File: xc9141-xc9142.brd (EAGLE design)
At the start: 13.6 x 21.6 mm, 7 parts

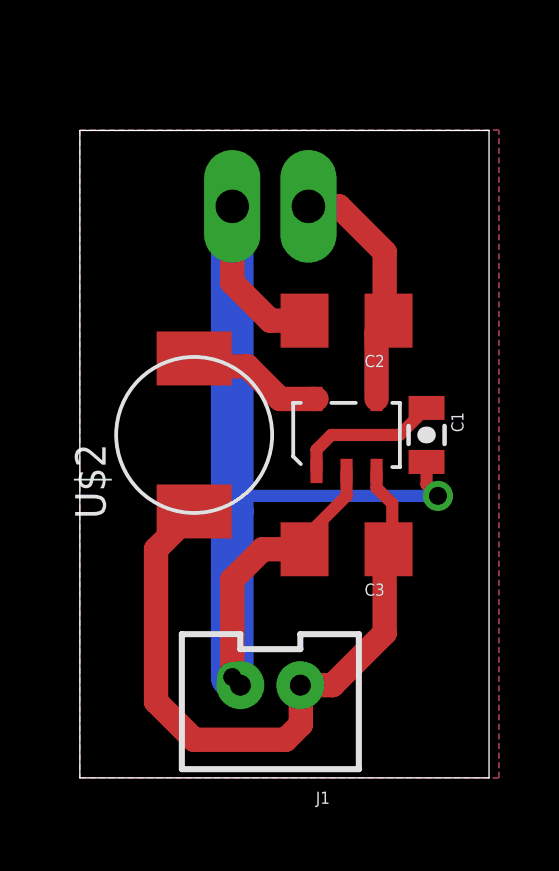
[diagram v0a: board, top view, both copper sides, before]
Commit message: Breakout board updates
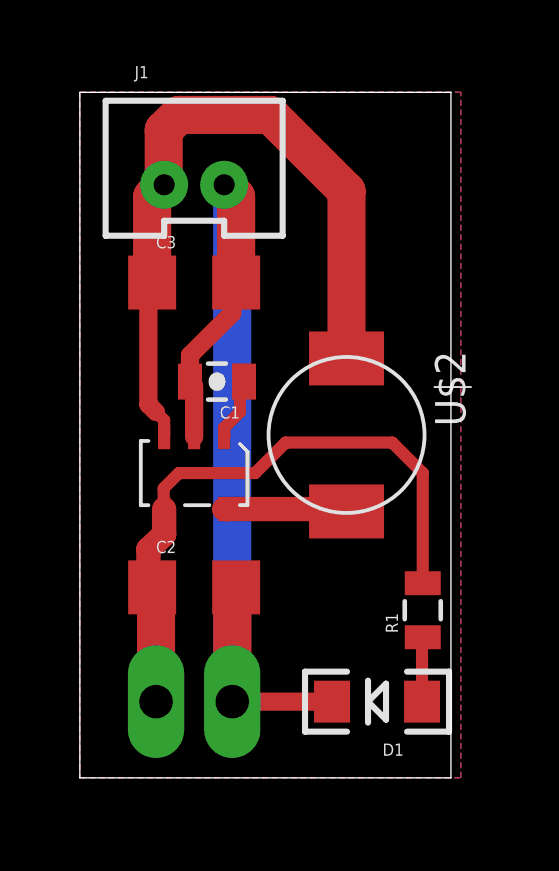
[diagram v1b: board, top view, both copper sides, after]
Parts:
- added D1: YELLOW, SparkFun-LED:LED-1206
- added R1: 680, SparkFun-Resistors:0805
- moved J1 18.0 mm to (3.81, 20.3), turned to 0 degrees
- moved J2 17.3 mm to (2.54, 2.54), turned to 0 degrees
- moved C2 10.2 mm to (3.81, 6.35), turned to 0 degrees
- moved C3 10.2 mm to (3.81, 16.5), turned to 0 degrees
- moved C1 7.21 mm to (4.57, 13.2), turned to 180 degrees
- moved U$1 5.24 mm to (3.81, 10.2), turned to 180 degrees
- moved U$2 5.08 mm to (8.89, 11.4), turned to 270 degrees
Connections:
- new net N$1: D1.A, R1.1
- net 5V: now also R1.2
- net GND: now also D1.C
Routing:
- net 5V: track 8.29 -> 20.8 mm
- net GND: track 39.2 -> 33.8 mm, vias 2 -> 0
- net N$2: track 4.95 -> 2.12 mm
- net N$1: track 0.00 -> 2.21 mm
- net V_BATT: track 23.0 -> 23.6 mm
- net N$4: track 4.64 -> 4.11 mm
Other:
- board size 13.6 x 21.6 mm -> 12.4 x 22.9 mm
